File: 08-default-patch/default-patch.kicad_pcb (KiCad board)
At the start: 2 copper layers, 210.7 x 32.5 mm, 30 parts

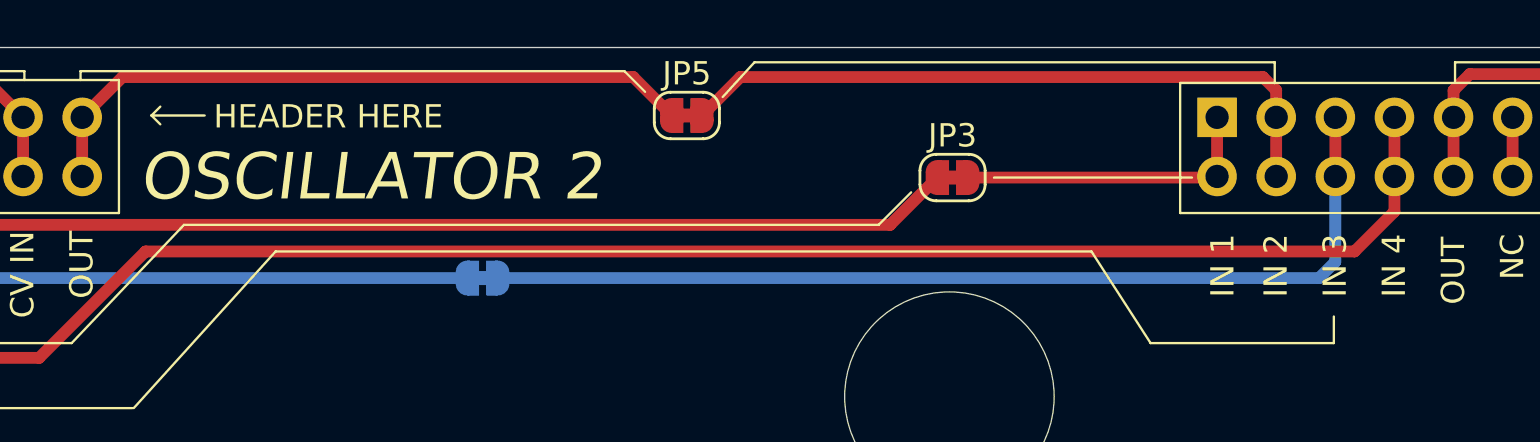
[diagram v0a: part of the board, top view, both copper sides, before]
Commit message: Reverted default patch
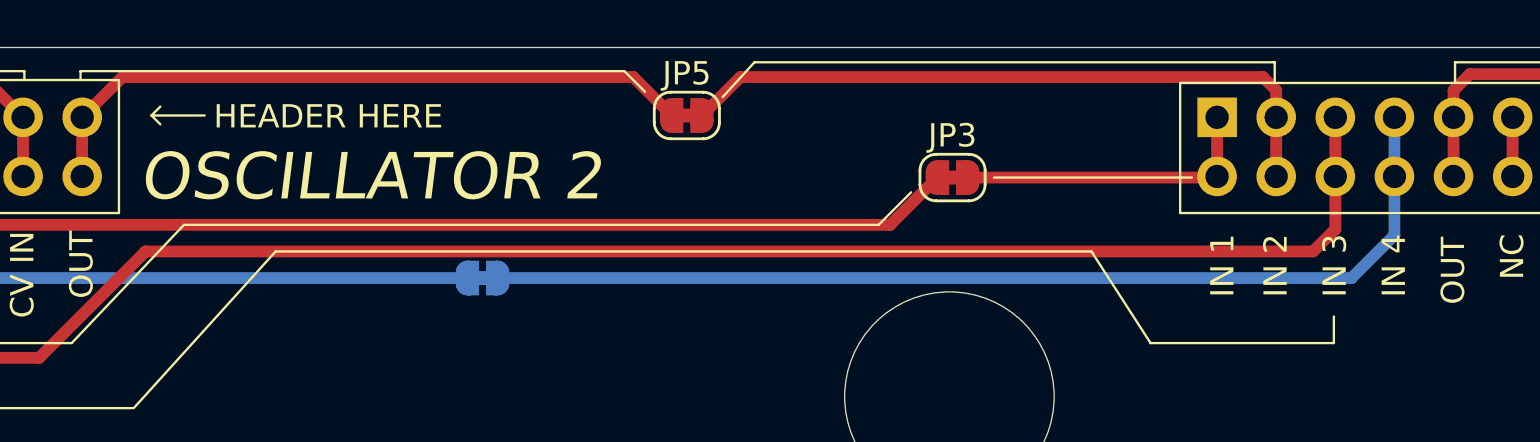
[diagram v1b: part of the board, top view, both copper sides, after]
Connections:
- J_MIXER1 pad 5: Net-(JP6-B) -> Net-(JP4-B)
- J_MIXER1 pad 6: Net-(JP6-B) -> Net-(JP4-B)
- J_MIXER1 pad 7: Net-(JP4-B) -> Net-(JP6-B)
- J_MIXER1 pad 8: Net-(JP4-B) -> Net-(JP6-B)
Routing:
- net Net-(JP4-B): track 100.9 -> 98.8 mm
- net Net-(JP6-B): track 42.5 -> 44.4 mm
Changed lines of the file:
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@@
 			(layers "*.Cu" "*.Mask")
 			(remove_unused_layers no)
-			(net 29 "Net-(JP6-B)")
+			(net 26 "Net-(JP4-B)")
 			(pinfunction "Pin_5")
 			(pintype "passive")
@@
 			(layers "*.Cu" "*.Mask")
 			(remove_unused_layers no)
-			(net 29 "Net-(JP6-B)")
+			(net 26 "Net-(JP4-B)")
 			(pinfunction "Pin_6")
 			(pintype "passive")
@@
 			(layers "*.Cu" "*.Mask")
 			(remove_unused_layers no)
-			(net 26 "Net-(JP4-B)")
+			(net 29 "Net-(JP6-B)")
 			(pinfunction "Pin_7")
 			(pintype "passive")
@@
 			(layers "*.Cu" "*.Mask")
 			(remove_unused_layers no)
-			(net 26 "Net-(JP4-B)")
+			(net 29 "Net-(JP6-B)")
 			(pinfunction "Pin_8")
 			(pintype "passive")
@@
 	)
 	(segment
-		(start 198.62 67.049)
-		(end 198.62 65.54)
+		(start 196.08 65.54)
+		(end 196.08 63)
 		(width 0.508)
 		(layer "F.Cu")
@@
 	)
 	(segment
-		(start 198.62 63)
-		(end 198.62 65.54)
+		(start 195.128 68.763)
+		(end 196.08 67.811)
 		(width 0.508)
 		(layer "F.Cu")
@@
 	)
 	(segment
-		(start 196.906 68.763)
-		(end 198.62 67.049)
+		(start 196.08 67.811)
+		(end 196.08 65.54)
 		(width 0.508)
 		(layer "F.Cu")
@@
 	(segment
 		(start 144.963 68.763)
-		(end 196.906 68.763)
+		(end 195.128 68.763)
 		(width 0.508)
 		(layer "F.Cu")
@@
 	)
 	(segment
-		(start 196.08 65.54)
-		(end 196.08 63)
-		(width 0.508)
-		(layer "F.Cu")
-		(net 29)
-	)
-	(segment
-		(start 196.08 69.208)
-		(end 196.08 65.54)
+		(start 198.62 68.065)
+		(end 198.62 63)
 		(width 0.508)
 		(layer "B.Cu")
@@
 	)
 	(segment
-		(start 160.091 69.906)
-		(end 195.382 69.906)
+		(start 196.779 69.906)
+		(end 198.62 68.065)
 		(width 0.508)
 		(layer "B.Cu")
@@
 	)
 	(segment
-		(start 195.382 69.906)
-		(end 196.08 69.208)
+		(start 160.091 69.906)
+		(end 196.779 69.906)
 		(width 0.508)
 		(layer "B.Cu")
